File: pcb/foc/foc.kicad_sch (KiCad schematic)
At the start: 34 parts, among them J1 PH_2.0, J2 TB_MOTOR, Q1 BTN8982TA, Q2 BTN8982TA, Q3 BTN8982TA, U1 INA240A2PW, U2 INA240A2PW

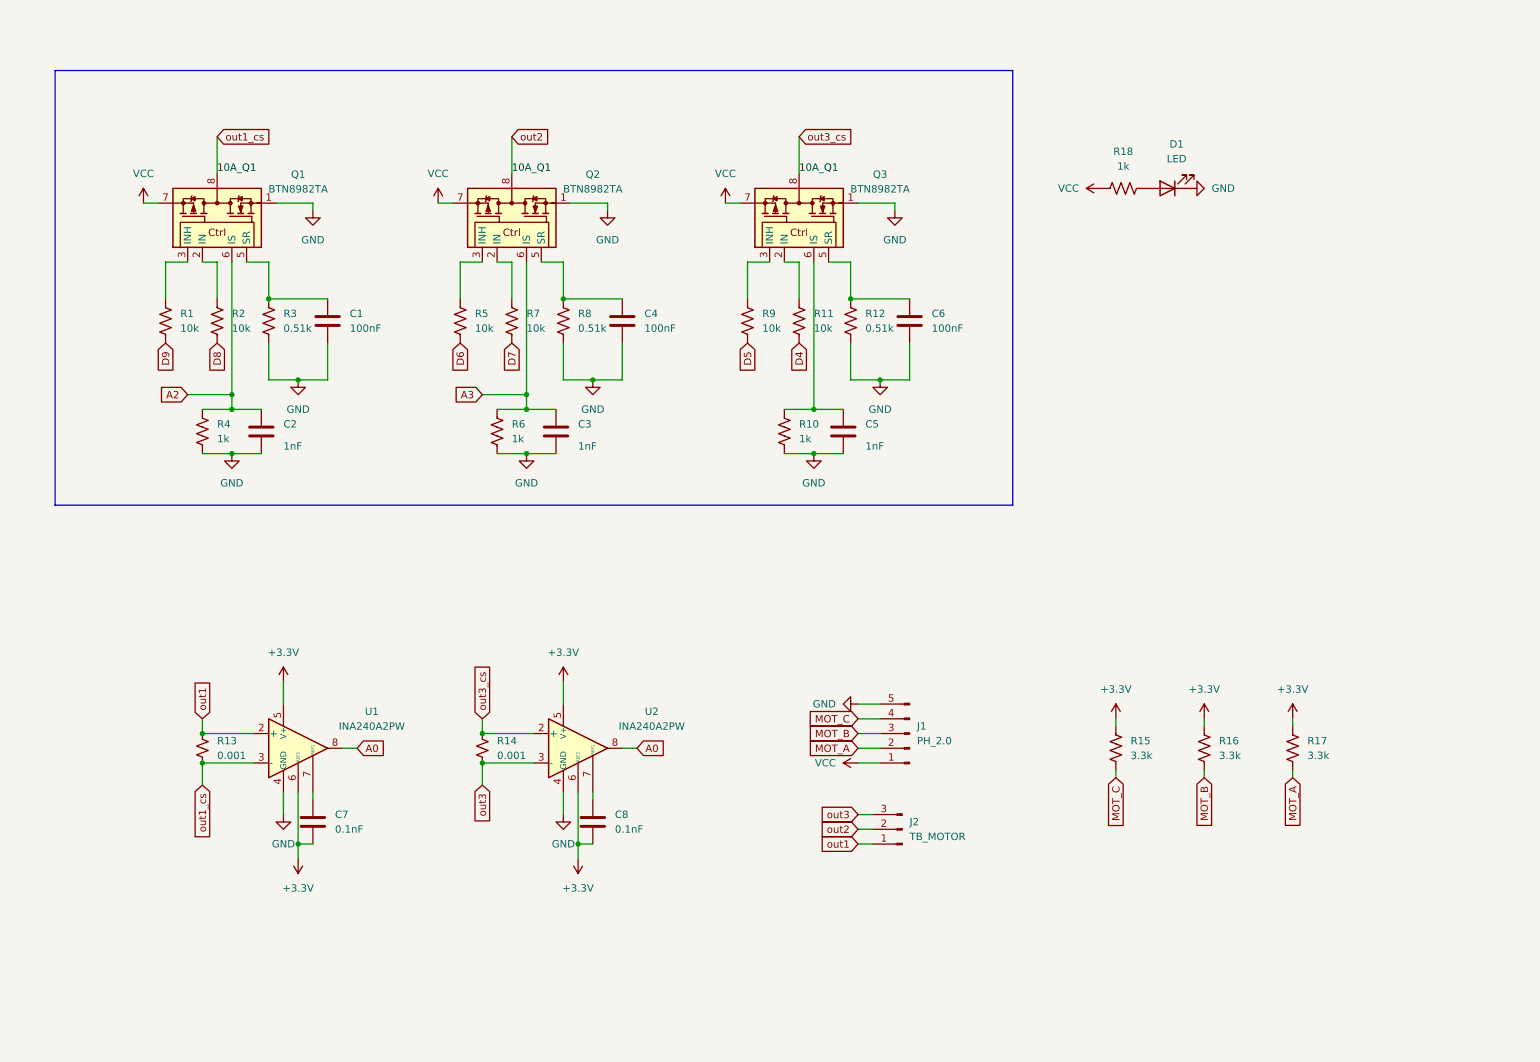
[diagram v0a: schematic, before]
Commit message: foc debug info designe
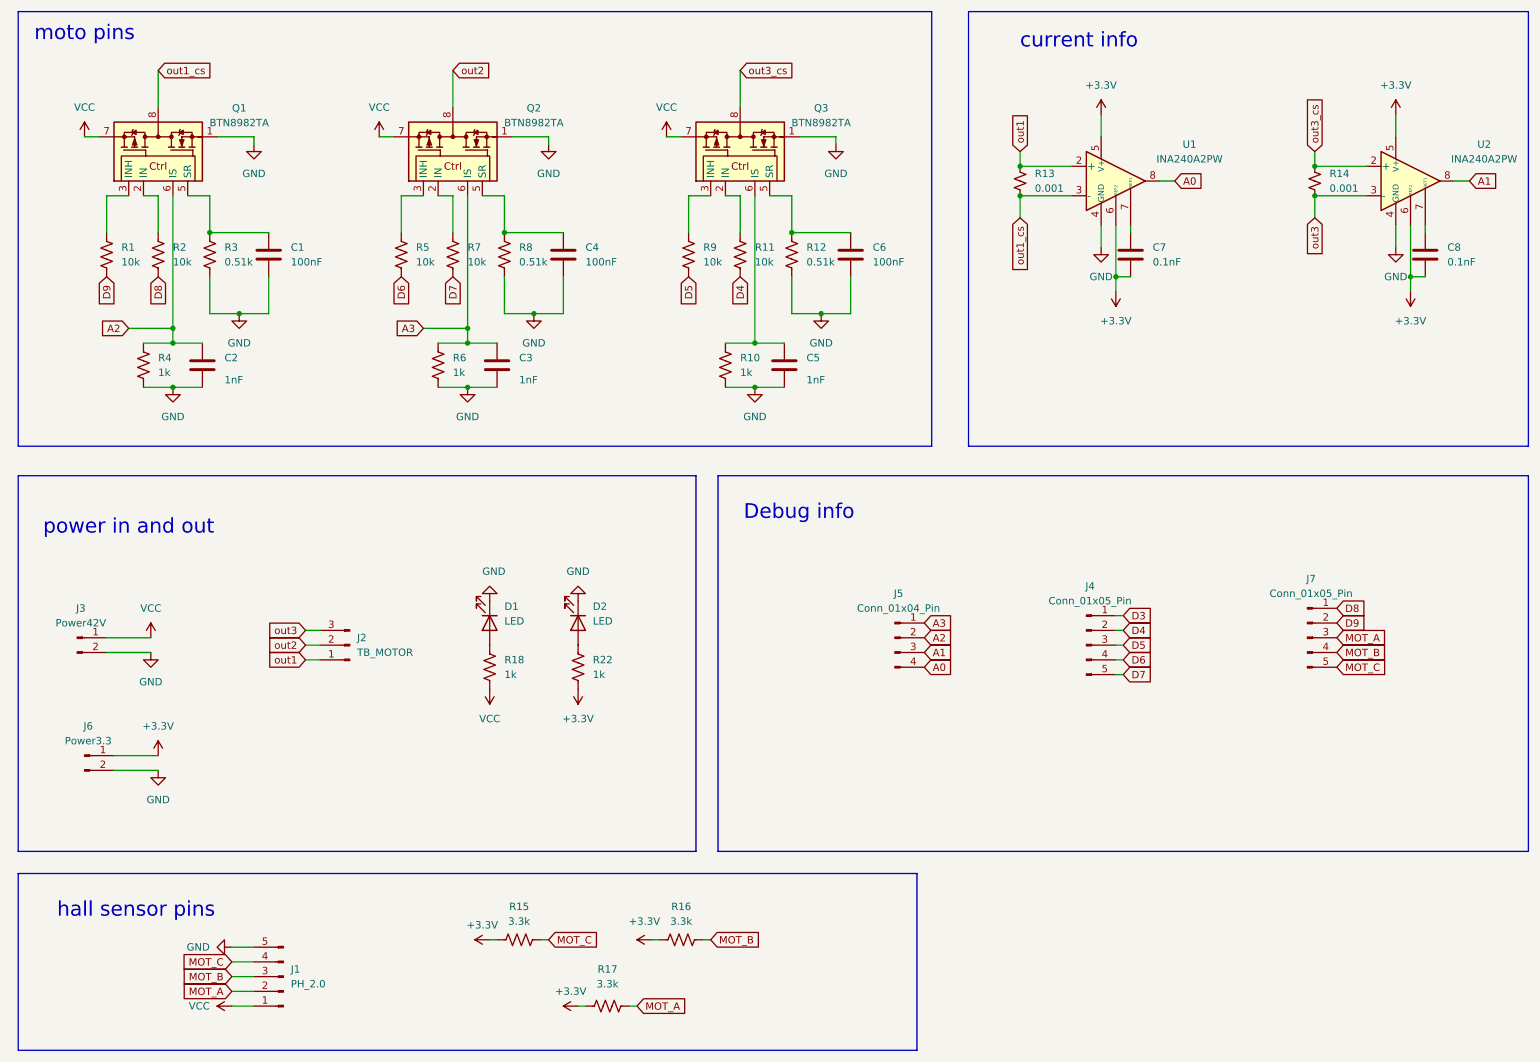
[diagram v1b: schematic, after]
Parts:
- added D2: LED, symbol Device:LED
- added J3: Power42V, symbol Connector:Conn_01x02_Pin
- added J4, J7: Conn_01x05_Pin, symbol Connector:Conn_01x05_Pin
- added J5: Conn_01x04_Pin, symbol Connector:Conn_01x04_Pin
- added J6: Power3.3, symbol Connector:Conn_01x02_Pin
- added R22: 1k, symbol Device:R_US
- R13, R14: footprint (none) -> Resistor_SMD:R_2512_6332Metric
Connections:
- net +3.3V: now also R15.2, R16.2, J6.1 (Pin_1), R22.2; no longer R15.1, R16.1
- net A0: now also J5.4 (Pin_4); no longer U2.8
- net A2: now also J5.2 (Pin_2)
- net A3: now also J5.1 (Pin_1)
- net D4: now also J4.2 (Pin_2)
- net D5: now also J4.3 (Pin_3)
- net D6: now also J4.4 (Pin_4)
- net D7: now also J4.5 (Pin_5)
- net D8: now also J7.1 (Pin_1)
- net D9: now also J7.2 (Pin_2)
- net GND: now also D2.1 (K), J3.2 (Pin_2), J6.2 (Pin_2)
- net MOT_A: now also J7.3 (Pin_3)
- net MOT_B: now also R16.1, J7.4 (Pin_4); no longer R16.2
- net MOT_C: now also R15.1, J7.5 (Pin_5); no longer R15.2
- net VCC: now also J3.1 (Pin_1)
- net out1_cs: no longer J2.2 (Pin_2), Q2.4, Q2.8, Q3.4, Q3.8, R14.1, U2.2 (+)
- new net: D2.2 (A), R22.1
- new net A1: J5.3 (Pin_3), U2.8
- new net D3: J4.1 (Pin_1)
- new net out2: J2.2 (Pin_2), Q2.4, Q2.8
- new net out3_cs: Q3.4, Q3.8, R14.1, U2.2 (+)
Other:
- note added: "Debug info"
- note added: "current info"
- note added: "hall sensor pins"
- note added: "moto pins"
- note added: "power in and out"
- moved on the sheet: C1, C2, C3, C4, C5, C6, C7, C8, D1, J1, J2, Q1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
